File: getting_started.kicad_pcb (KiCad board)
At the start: 2 copper layers, 37 x 13 mm, 13 parts, among them J1 Prog connector, J2 Conn_01x03_Pin, U1 STM32F030F4Px, U2 SHT4x

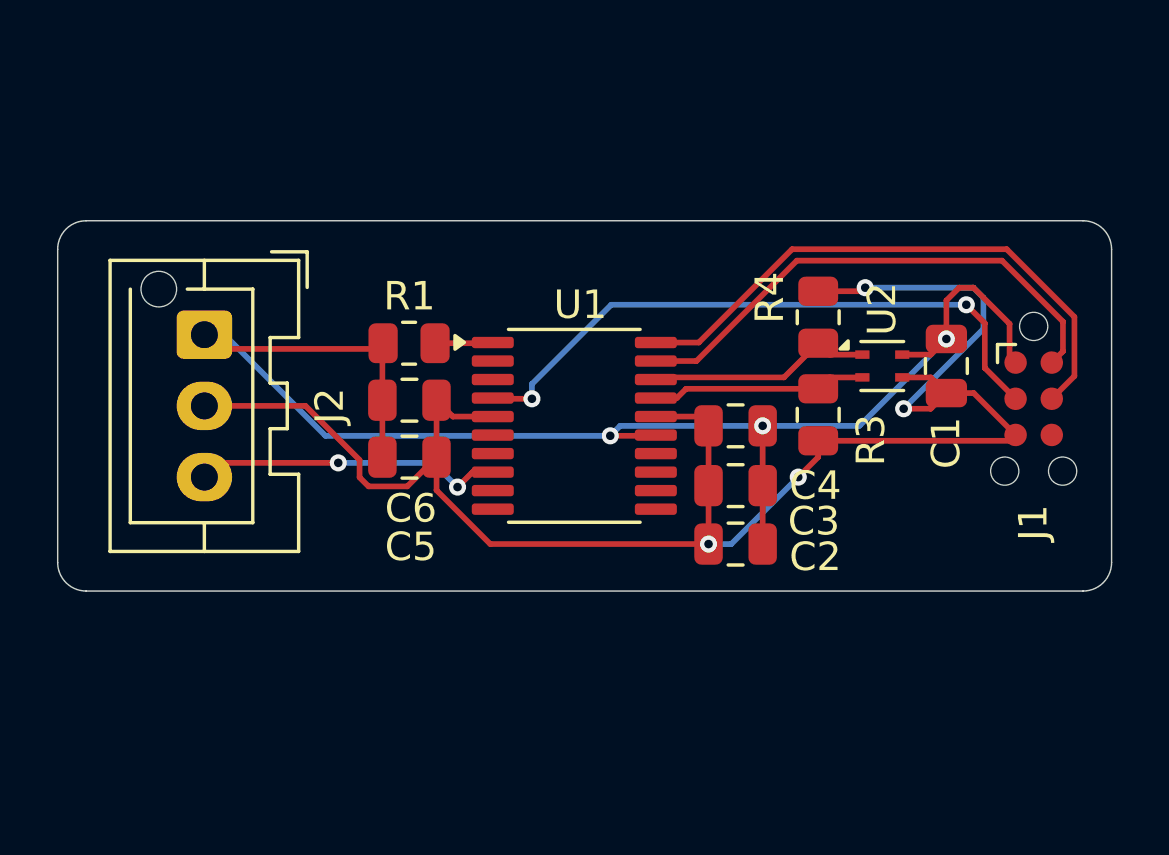
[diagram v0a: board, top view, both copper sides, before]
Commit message: Updated schematic and pcb
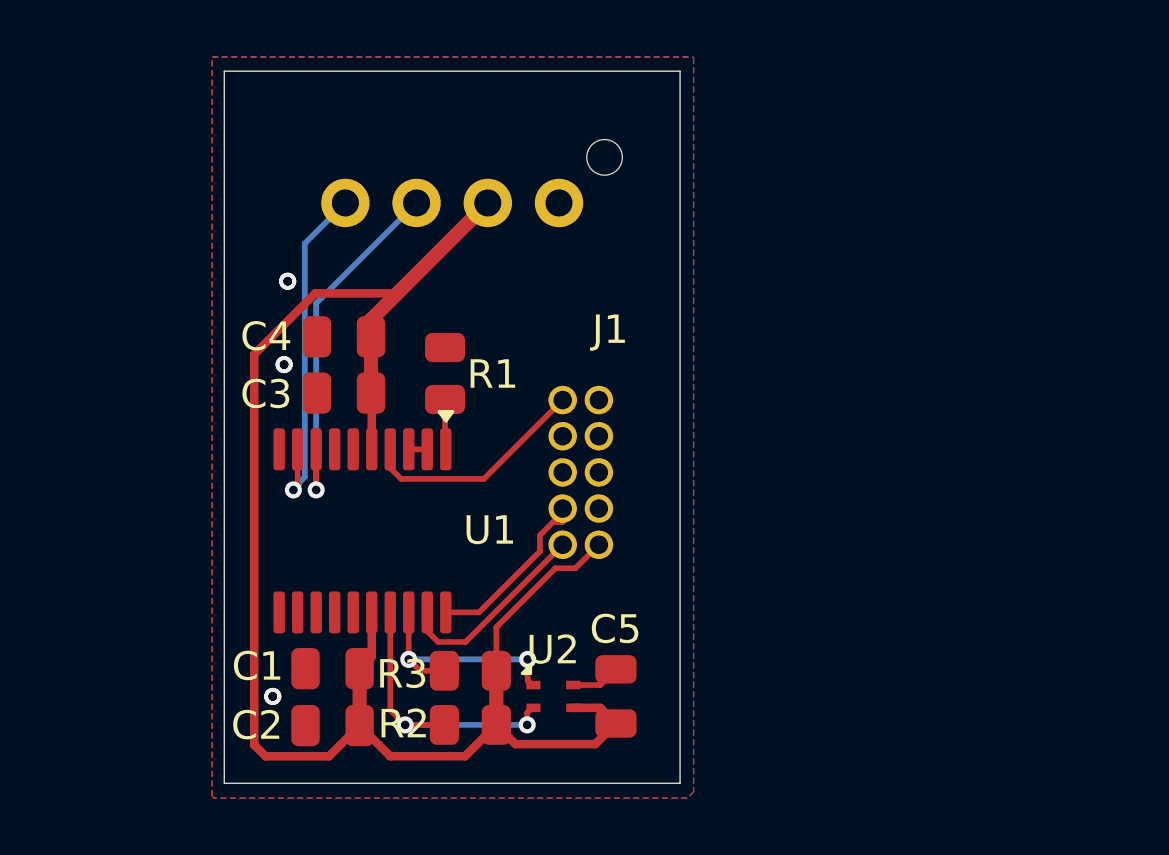
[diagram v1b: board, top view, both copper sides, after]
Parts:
- removed the C4 at (122.0, 113.0)
- J1: value Prog connector -> Conn_01x04_Pin; footprint Connector:Tag-Connect_TC2030-IDC-NL_2x03_P1.27mm_Vertical -> Connector_JST:JST_XA_B04B-XASK-1-A_1x04_P2.50mm_Vertical
- J2: value Conn_01x03_Pin -> Conn_ARM_JTAG_SWD_10; footprint Connector_JST:JST_XA_B03B-XASK-1-A_1x03_P2.50mm_Vertical -> Connector_PinHeader_1.27mm:PinHeader_2x05_P1.27mm_Vertical
- moved J1 18.0 mm to (115.8, 105.1), turned to 180 degrees
- moved R3 17.4 mm to (112.6, 121.5), turned to 180 degrees
- moved C2 16.5 mm to (107.8, 123.5), turned to 180 degrees
- moved C5 16.4 mm to (117.8, 122.5)
- moved U2 16.4 mm to (115.5, 122.5)
- moved R2 16.4 mm to (112.6, 123.5), turned to 180 degrees
- moved J2 15.7 mm to (117.2, 117.1), turned to 180 degrees
- moved C1 14.8 mm to (107.8, 121.5), turned to 180 degrees
- moved U1 8.30 mm to (108.8, 116.6), turned to -90 degrees
- moved C3 3.22 mm to (108.2, 111.8)
- moved C4 3.20 mm to (108.2, 109.8)
- moved R1 1.65 mm to (111.8, 111.1), turned to 90 degrees
- renumbered C3 to C1, C5 to C3, C6 to C4, C1 to C5, R3 to R2, R4 to R3
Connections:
- J1 pad 2: /SWDIO -> +3.3V
- J1 pad 3: /nReset -> /IO_TX
- J1 pad 4: /SWCLK -> /IO_RX
- J2 pad 1: GND -> +3.3V
- J2 pad 2: +3.3V -> /SWDIO
- J2 pad 3: /IO -> GND
- U1 pad 10: unconnected-(U1-PA4-Pad10) -> GND
- U1 pad 11: unconnected-(U1-PA5-Pad11) -> GND
- U1 pad 12: unconnected-(U1-PA6-Pad12) -> GND
- U1 pad 13: unconnected-(U1-PA7-Pad13) -> GND
- U1 pad 14: unconnected-(U1-PB1-Pad14) -> GND
- U1 pad 2: unconnected-(U1-PF0-Pad2) -> GND
- U1 pad 3: unconnected-(U1-PF1-Pad3) -> GND
- U1 pad 4: /nReset -> /nRESET
- U1 pad 6: unconnected-(U1-PA0-Pad6) -> GND
- U1 pad 7: unconnected-(U1-PA1-Pad7) -> GND
- U1 pad 8: /IO -> /IO_TX
- U1 pad 9: unconnected-(U1-PA3-Pad9) -> /IO_RX
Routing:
- net GND: track 52.8 -> 2.45 mm, vias 3 -> 6
- net /nReset: track 22.3 -> 0.00 mm, vias 2 -> 0
- net /SWCLK: track 20.2 -> 6.22 mm
- net /IO_TX: track 0.00 -> 13.0 mm, vias 0 -> 1
- net /IO_RX: track 0.00 -> 12.3 mm, vias 0 -> 1
- net /SWDIO: track 18.2 -> 6.98 mm
- net /IO: track 10.9 -> 0.00 mm, vias 2 -> 0
- net /nRESET: track 0.00 -> 8.05 mm
- net +3.3V: track 62.3 -> 58.9 mm, vias 4 -> 0
- net Net-(U1-PA9): track 7.55 -> 10.5 mm, vias 0 -> 2
- net Net-(U1-PA10): track 7.94 -> 8.36 mm, vias 0 -> 2
- added copper zone on B.Cu, net GND
- added copper zone on F.Cu, net GND
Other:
- board size 37 x 13 mm -> 16 x 25 mm
